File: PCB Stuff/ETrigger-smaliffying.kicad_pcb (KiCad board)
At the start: 2 copper layers, 33.7 x 27.5 mm, 51 parts, among them IC1 ATTINY85-S, P1 CONN_01X04

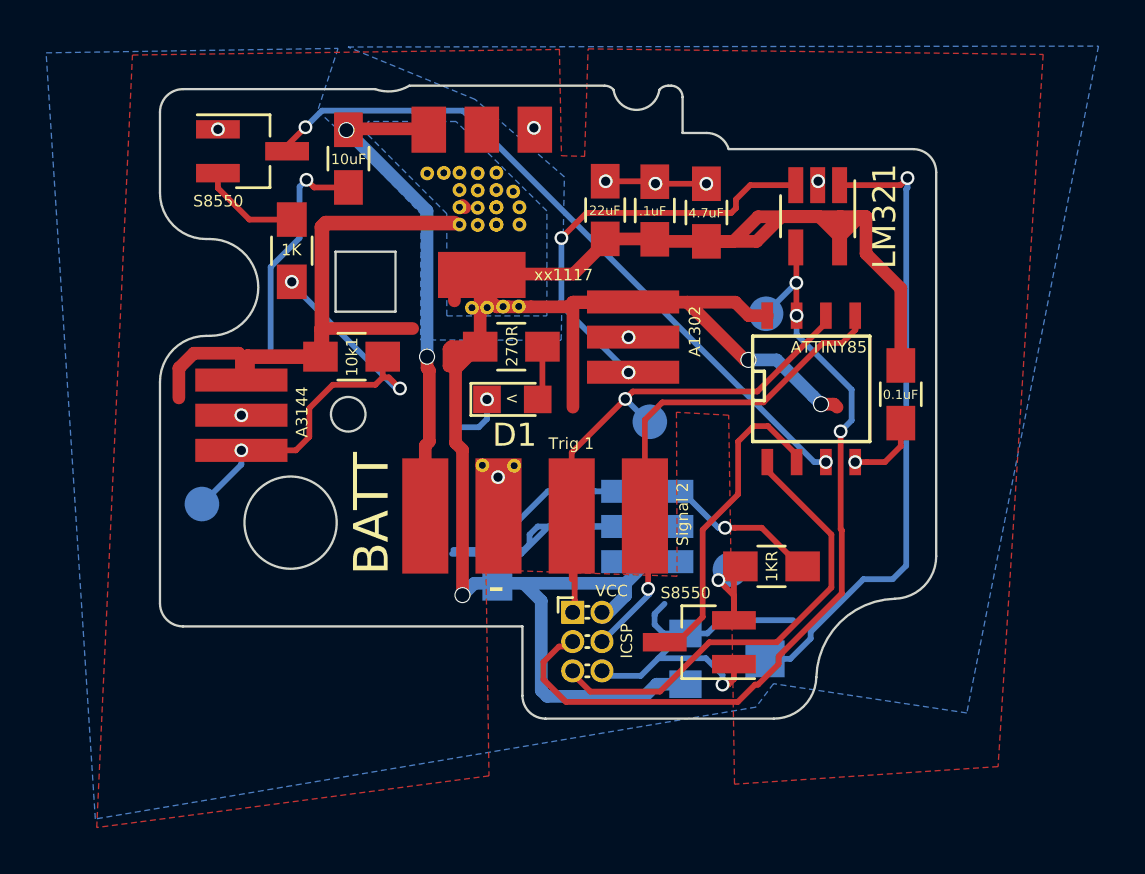
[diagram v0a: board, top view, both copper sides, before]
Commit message: Revert "Small Changes Already..."
This reverts commit acef30372dc182f28b0b01e172afb46279e9fedb.
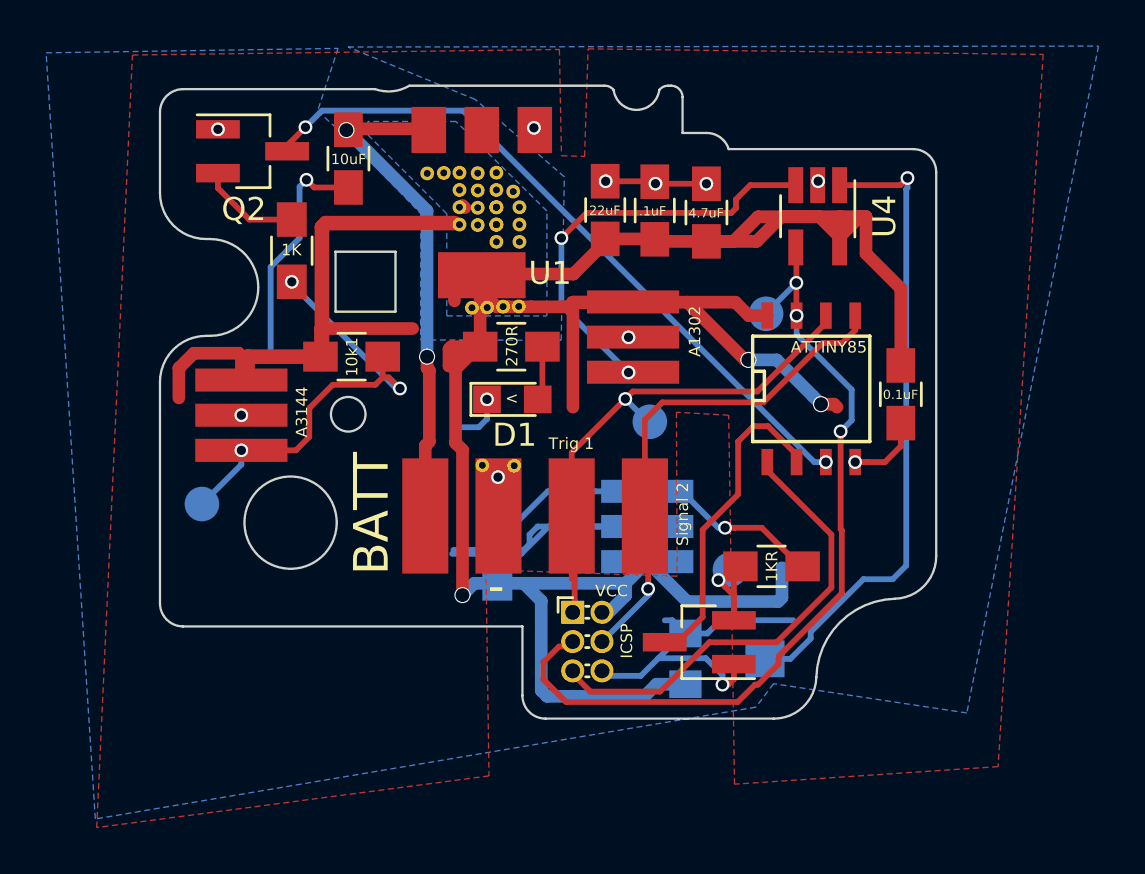
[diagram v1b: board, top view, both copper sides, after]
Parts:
- added REF**: Via 2, Via 2, F.Cu at (152.5, 90.8)
- added REF**: Via 2, Via 2, F.Cu at (151.5, 90.8)
- renumbered S8550 to Q1, S8550 to Q2, xx1117 to U1, LM321 to U4
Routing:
- net VCC_ICSP: track 132.7 -> 140.6 mm
- net GND_ICSP: track 57.8 -> 56.4 mm
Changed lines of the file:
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@@
 (kicad_pcb (version 4) (host pcbnew 4.0.5)
   (general
-    (links 0)
+    (links 82)
     (no_connects 0)
     (area 136.830709 82.456999 170.595002 111.507001)
     (thickness 1.6)
     (drawings 248)
-    (tracks 318)
+    (tracks 319)
     (zones 0)
-    (modules 51)
+    (modules 53)
     (nets 17)
   )
   (page A4)
   (layers
-    (0 F.Cu signal hide)
+    (0 F.Cu signal)
     (31 B.Cu signal)
     (32 B.Adhes user)
@@
     (visible_elements 7FFEF6FF)
     (pcbplotparams
-      (layerselection 0x011f0_80000001)
-      (usegerberextensions true)
+      (layerselection 0x00030_80000001)
+      (usegerberextensions false)
       (excludeedgelayer true)
       (linewidth 0.100000)
@@
       (outputformat 1)
       (mirror false)
-      (drillshape 0)
+      (drillshape 1)
       (scaleselection 1)
-      (outputdirectory "ETrig Board/"))
+      (outputdirectory ""))
   )
   (net 0 "")
@@
     (add_net VCC_ICSP)
   )
-  (module TO_SOT_Packages_SMD:SOT-223 (layer F.Cu)
-    (at 150.8379 89.0647 270)
-    (descr "module CMS SOT223 4 pins")
-    (tags "CMS SOT")
-    (attr smd)
-    (fp_text reference xx1117 (at 3.15 -3.5433 360) (layer F.SilkS)
-      (effects (font (size 0.5 0.5) (thickness 0.1)))
-    )
-    (fp_text value AP1117 (at 0 4.5 270) (layer F.Fab)
-      (effects (font (size 1 1) (thickness 0.15)))
-    )
-    (fp_text user %R (at 0 0 270) (layer F.Fab)
-      (effects (font (size 0.8 0.8) (thickness 0.12)))
-    )
-    (fp_line (start -1.85 -2.3) (end -0.8 -3.35) (layer F.Fab) (width 0.1))
-    (fp_line (start 4.4 -3.6) (end -4.4 -3.6) (layer F.CrtYd) (width 0.05))
-    (fp_line (start 4.4 3.6) (end 4.4 -3.6) (layer F.CrtYd) (width 0.05))
-    (fp_line (start -4.4 3.6) (end 4.4 3.6) (layer F.CrtYd) (width 0.05))
-    (fp_line (start -4.4 -3.6) (end -4.4 3.6) (layer F.CrtYd) (width 0.05))
-    (fp_line (start -1.85 -2.3) (end -1.85 3.35) (layer F.Fab) (width 0.1))
-    (fp_line (start -0.8 -3.35) (end 1.85 -3.35) (layer F.Fab) (width 0.1))
-    (fp_line (start -1.85 3.35) (end 1.85 3.35) (layer F.Fab) (width 0.1))
-    (fp_line (start 1.85 -3.35) (end 1.85 3.35) (layer F.Fab) (width 0.1))
-    (pad 4 smd rect (at 3.15 0 270) (size 2 3.8) (layers *.Mask F.Cu F.Paste)
-      (net 1 VCC_ICSP) (zone_connect 2))
-    (pad 2 smd rect (at -3.15 0 270) (size 2 1.5) (layers *.Mask F.Cu F.Paste)
-      (net 1 VCC_ICSP))
-    (pad 3 smd rect (at -3.15 2.3 270) (size 2 1.5) (layers *.Mask F.Cu F.Paste)
-      (net 4 +BATT))
-    (pad 1 smd rect (at -3.15 -2.3 270) (size 2 1.5) (layers *.Mask F.Cu F.Paste)
-      (net 5 GND_ICSP))
-    (model ${KISYS3DMOD}/TO_SOT_Packages_SMD.3dshapes/SOT-223.wrl
-      (at (xyz 0 0 0))
-      (scale (xyz 0.5 0.5 0.5))
-      (rotate (xyz 0 0 90))
-    )
-  )
   (module Capacitors_SMD:C_0805_HandSoldering (layer F.Cu)
     (at 169.01 97.39 270)
@@
   )
   (module "Via 2" (layer F.Cu)
+    (at 152.47 90.78)
+    (clearance 0.00001)
+    (zone_connect 2)
+    (fp_text reference REF** (at 0.127 4.699) (layer F.SilkS) hide
+      (effects (font (size 0.127 0.127) (thickness 0.03175)))
+    )
+    (fp_text value "Via 2" (at -0.127 -5.969) (layer F.Fab) hide
+      (effects (font (size 0.127 0.127) (thickness 0.03175)))
+    )
+    (pad 1 thru_hole circle (at 0 0) (size 0.6 0.6) (drill 0.3) (layers *.Cu)
+      (net 1 VCC_ICSP) (zone_connect 2))
+  )
+  (module "Via 2" (layer F.Cu)
+    (at 151.47 90.78)
+    (clearance 0.00001)
+    (zone_connect 2)
+    (fp_text reference REF** (at 0.127 4.699) (layer F.SilkS) hide
+      (effects (font (size 0.127 0.127) (thickness 0.03175)))
+    )
+    (fp_text value "Via 2" (at -0.127 -5.969) (layer F.Fab) hide
+      (effects (font (size 0.127 0.127) (thickness 0.03175)))
+    )
+    (pad 1 thru_hole circle (at 0 0) (size 0.6 0.6) (drill 0.3) (layers *.Cu)
+      (net 1 VCC_ICSP) (zone_connect 2))
+  )
+  (module "Via 2" (layer F.Cu)
     (at 152.47 90.03)
     (clearance 0.00001)
@@
     (pad 1 thru_hole circle (at 0 0) (size 0.6 0.6) (drill 0.3) (layers *.Cu)
       (net 5 GND_ICSP) (zone_connect 2))
+  )
+  (module TO_SOT_Packages_SMD:SOT-223 (layer F.Cu)
+    (at 150.8379 89.0774 270)
+    (descr "module CMS SOT223 4 pins")
+    (tags "CMS SOT")
+    (attr smd)
+    (fp_text reference U1 (at 3.0611 -2.9591 360) (layer F.SilkS)
+      (effects (font (size 1 1) (thickness 0.15)))
+    )
+    (fp_text value AP1117 (at 0 4.5 270) (layer F.Fab)
+      (effects (font (size 1 1) (thickness 0.15)))
+    )
+    (fp_text user %R (at 0 0 270) (layer F.Fab)
+      (effects (font (size 0.8 0.8) (thickness 0.12)))
+    )
+    (fp_line (start -1.85 -2.3) (end -0.8 -3.35) (layer F.Fab) (width 0.1))
+    (fp_line (start 4.4 -3.6) (end -4.4 -3.6) (layer F.CrtYd) (width 0.05))
+    (fp_line (start 4.4 3.6) (end 4.4 -3.6) (layer F.CrtYd) (width 0.05))
+    (fp_line (start -4.4 3.6) (end 4.4 3.6) (layer F.CrtYd) (width 0.05))
+    (fp_line (start -4.4 -3.6) (end -4.4 3.6) (layer F.CrtYd) (width 0.05))
+    (fp_line (start -1.85 -2.3) (end -1.85 3.35) (layer F.Fab) (width 0.1))
+    (fp_line (start -0.8 -3.35) (end 1.85 -3.35) (layer F.Fab) (width 0.1))
+    (fp_line (start -1.85 3.35) (end 1.85 3.35) (layer F.Fab) (width 0.1))
+    (fp_line (start 1.85 -3.35) (end 1.85 3.35) (layer F.Fab) (width 0.1))
+    (pad 4 smd rect (at 3.15 0 270) (size 2 3.8) (layers F.Cu F.Paste)
+      (net 1 VCC_ICSP) (zone_connect 2))
+    (pad 2 smd rect (at -3.15 0 270) (size 2 1.5) (layers F.Cu F.Paste)
+      (net 1 VCC_ICSP))
+    (pad 3 smd rect (at -3.15 2.3 270) (size 2 1.5) (layers F.Cu F.Paste)
+      (net 4 +BATT))
+    (pad 1 smd rect (at -3.15 -2.3 270) (size 2 1.5) (layers F.Cu F.Paste)
+      (net 5 GND_ICSP))
+    (model ${KISYS3DMOD}/TO_SOT_Packages_SMD.3dshapes/SOT-223.wrl
+      (at (xyz 0 0 0))
+      (scale (xyz 0.5 0.5 0.5))
+      (rotate (xyz 0 0 90))
+    )
   )
   (module Via (layer F.Cu)
@@
     (tags "SOT-23-5 hand-soldering")
     (attr smd)
-    (fp_text reference LM321 (at 0 -2.9 270) (layer F.SilkS)
+    (fp_text reference U4 (at 0 -2.9 270) (layer F.SilkS)
       (effects (font (size 1 1) (thickness 0.15)))
     )
@@
     (tags SOT-23)
     (attr smd)
-    (fp_text reference S8550 (at 0.5955 2.13614 180) (layer F.SilkS)
-      (effects (font (size 0.5 0.5) (thickness 0.1)))
+    (fp_text reference Q1 (at 0 -2.5 180) (layer F.SilkS) hide
+      (effects (font (size 1 1) (thickness 0.15)))
     )
     (fp_text value S8550 (at 0 2.5 180) (layer F.Fab)
@@
       (at (xyz 0 0 0))
       (scale (xyz 1 1 1))
-      (rotate (xyz 0 0 90))
+      (rotate (xyz 0 0 0))
     )
   )
@@
     (tags SOT-23)
     (attr smd)
-    (fp_text reference S8550 (at -1.4859 2.16408) (layer F.SilkS)
-      (effects (font (size 0.5 0.5) (thickness 0.1)))
+    (fp_text reference Q2 (at -0.3738 2.51978) (layer F.SilkS)
+      (effects (font (size 1 1) (thickness 0.15)))
     )
     (fp_text value S8550 (at 0 2.5) (layer F.Fab)
@@
       (at (xyz 0 0 0))
       (scale (xyz 1 1 1))
-      (rotate (xyz 0 0 90))
+      (rotate (xyz 0 0 0))
     )
   )
@@
     (tags "Mesurement Point Round SMD Pad 1.5mm")
     (attr virtual)
-    (fp_text reference W4 (at 0.1091 -1.7617) (layer B.SilkS)
+    (fp_text reference W4 (at 0.04 -2.78) (layer B.SilkS)
       (effects (font (size 1 1) (thickness 0.15)) (justify mirror))
     )
@@
   (via (at 162.4 95.9) (size 0.7) (drill 0.6) (layers F.Cu B.Cu) (net 1))
   (segment (start 162.2548 95.9) (end 162.4 95.9) (width 0.55) (layer F.Cu) (net 1))
+  (segment (start 159.745317 106.379917) (end 158.0134 104.648) (width 0.55) (layer B.Cu) (net 1))
+  (segment (start 163.688283 106.379917) (end 159.745317 106.379917) (width 0.55) (layer B.Cu) (net 1))
+  (segment (start 163.8554 106.2128) (end 163.688283 106.379917) (width 0.55) (layer B.Cu) (net 1))
+  (segment (start 163.8554 104.9128) (end 163.8554 106.2128) (width 0.55) (layer B.Cu) (net 1))
   (segment (start 137.7 96.26) (end 137.7 97.55) (width 0.55) (layer F.Cu) (net 1))
   (segment (start 137.74 96.22) (end 137.7 96.26) (width 0.55) (layer F.Cu) (net 1))
@@
   (via (at 144.966145 85.934137) (size 0.7) (drill 0.6) (layers F.Cu B.Cu) (net 4))
   (via (at 148.463 95.758) (size 0.7) (drill 0.6) (layers F.Cu B.Cu) (net 4))
-  (segment (start 158.3309 106.9086) (end 158.7627 106.4768) (width 0.25) (layer B.Cu) (net 5))
-  (segment (start 158.3309 106.9975) (end 158.3309 106.9086) (width 0.25) (layer B.Cu) (net 5))
-  (segment (start 158.3309 107.3765) (end 158.3309 106.9975) (width 0.25) (layer B.Cu) (net 5))
-  (segment (start 159.6688 107.7644) (end 158.7188 107.7644) (width 0.25) (layer B.Cu) (net 5))
-  (segment (start 158.7188 107.7644) (end 158.3309 107.3765) (width 0.25) (layer B.Cu) (net 5))
   (segment (start 152.673615 85.835353) (end 153.097879 85.835353) (width 0.25) (layer F.Cu) (net 5))
   (segment (start 152.654847 85.835353) (end 152.673615 85.835353) (width 0.25) (layer F.Cu) (net 5))
@@
   (segment (start 151.5618 102.6668) (end 151.541135 102.646135) (width 0.25) (layer F.Cu) (net 5))
   (via (at 151.541135 100.983493) (size 0.6) (drill 0.4) (layers F.Cu B.Cu) (net 5))
+  (segment (start 158.7726 107.19304) (end 159.09744 107.19304) (width 0.25) (layer B.Cu) (net 5))
+  (segment (start 159.09744 107.19304) (end 159.6688 107.7644) (width 0.25) (layer B.Cu) (net 5))
   (via (at 139.3938 85.90022) (size 0.6) (drill 0.4) (layers F.Cu B.Cu) (net 5))
   (via (at 151.0636 97.6122) (size 0.6) (drill 0.4) (layers F.Cu B.Cu) (net 5))
@@
       )
     )
+  )
+  (zone (net 0) (net_name "") (layer F.Mask) (hatch edge 0.508)
+    (connect_pads (clearance 0.508))
+    (min_thickness 0.254)
+    (fill yes (arc_segments 16) (thermal_gap 0.508) (thermal_bridge_width 0.508))
+    (polygon
+      (pts
+        (xy 147.32 91.059) (xy 147.32 87.122) (xy 154.305 87.122) (xy 154.305 91.059)
+      )
+    )
